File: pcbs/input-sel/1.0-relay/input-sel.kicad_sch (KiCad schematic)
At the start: 54 parts, among them J1 Conn_01x03_Pin, J10 Conn_01x04_Pin, J2 Conn_01x03_Pin, J3 Conn_01x03_Pin, J4 Conn_01x03_Pin, J5 Conn_01x03_Pin, J6 Conn_01x03_Pin, J7 Conn_01x02_Pin, J8 Conn_01x02_Pin, J9 Conn_01x03_Pin, K1 EC2-5NU, K2 EC2-5NU, K3 EC2-5NU, K4 EC2-5NU, K5 EC2-5NU, K6 EC2-5NU, U1 CD74AC238, U2 TCMT4600, U3 TCMT4600

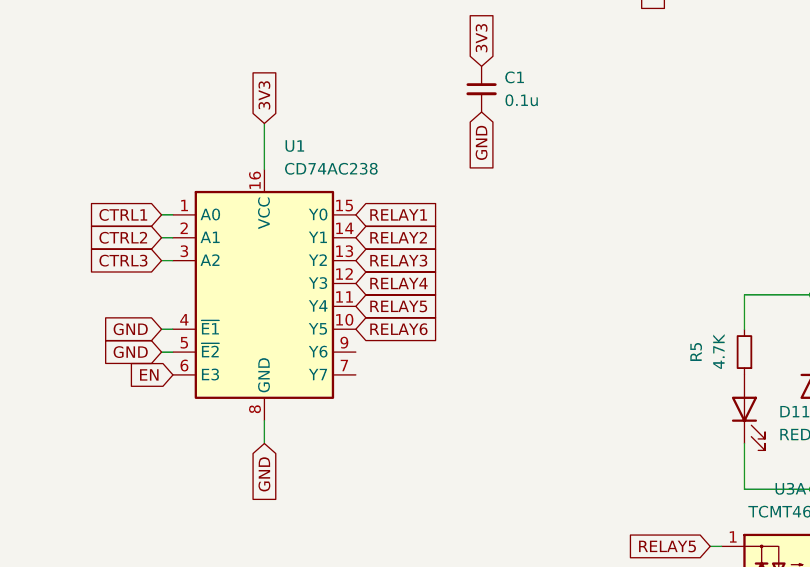
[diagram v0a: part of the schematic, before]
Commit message: Updates to pcbs
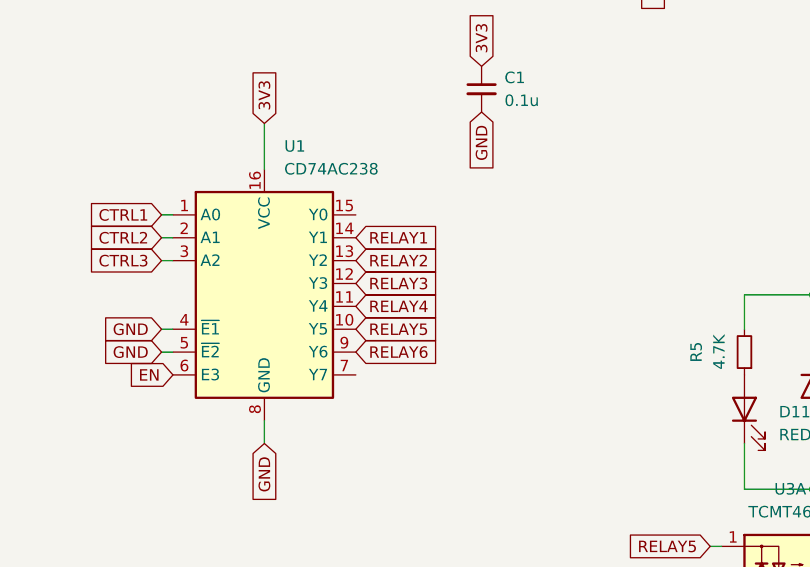
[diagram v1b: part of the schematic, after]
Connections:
- net RELAY1: now also U1.14 (Y1); no longer U1.15 (Y0)
- net RELAY2: now also U1.13 (Y2); no longer U1.14 (Y1)
- net RELAY3: now also U1.12 (Y3); no longer U1.13 (Y2)
- net RELAY4: now also U1.11 (Y4); no longer U1.12 (Y3)
- net RELAY5: now also U1.10 (Y5); no longer U1.11 (Y4)
- net RELAY6: now also U1.9 (Y6); no longer U1.10 (Y5)
